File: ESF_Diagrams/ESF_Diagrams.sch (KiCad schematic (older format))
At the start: 37 parts, among them M1 Motor, M2 Motor, U2 AIR, U3 AIR

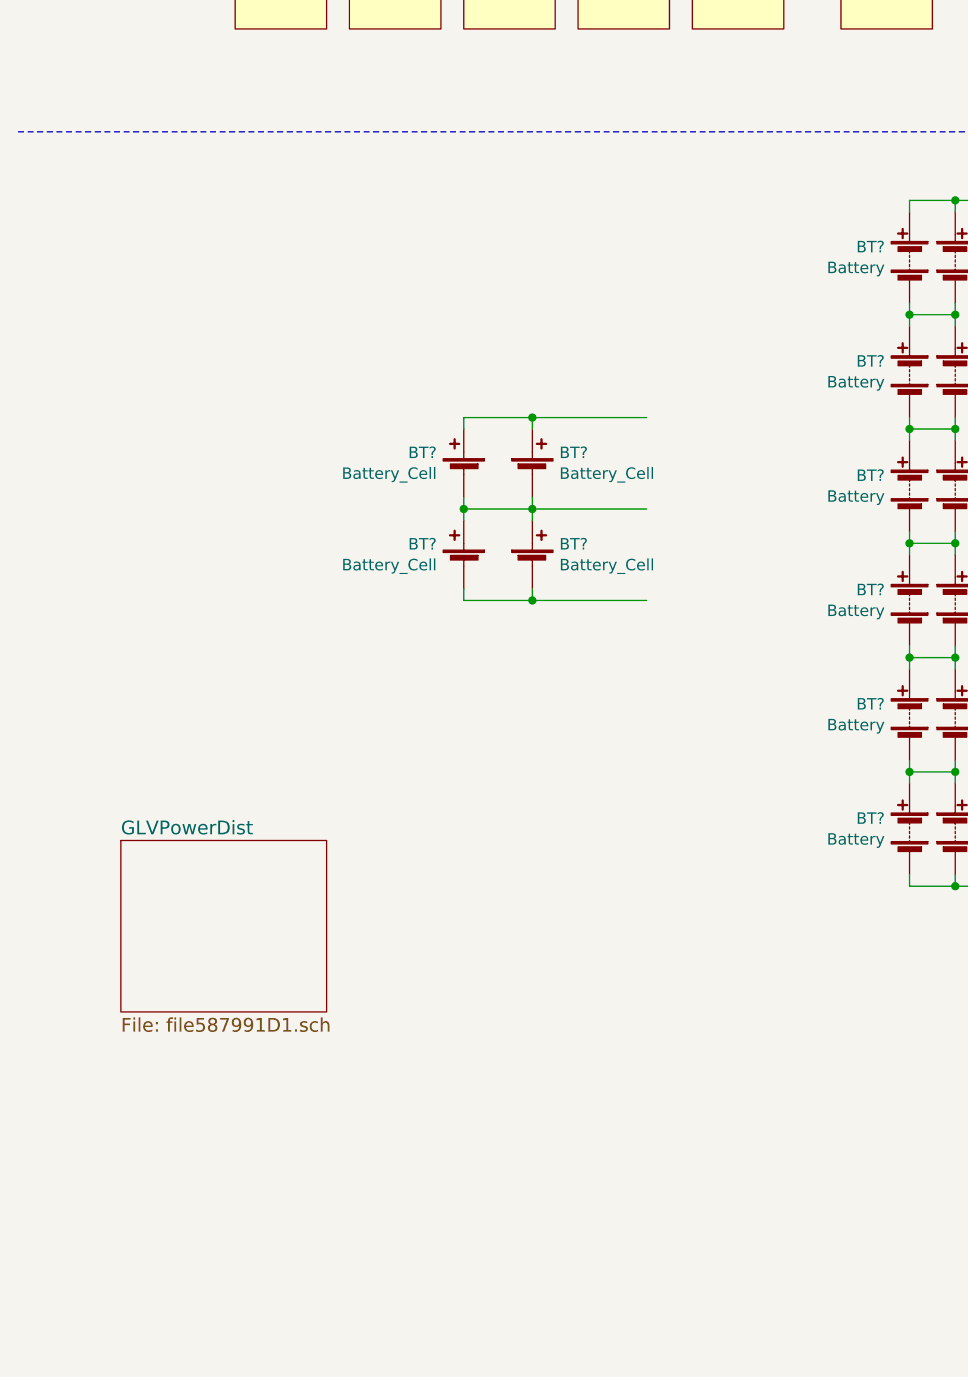
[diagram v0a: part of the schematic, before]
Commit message: Fix 2
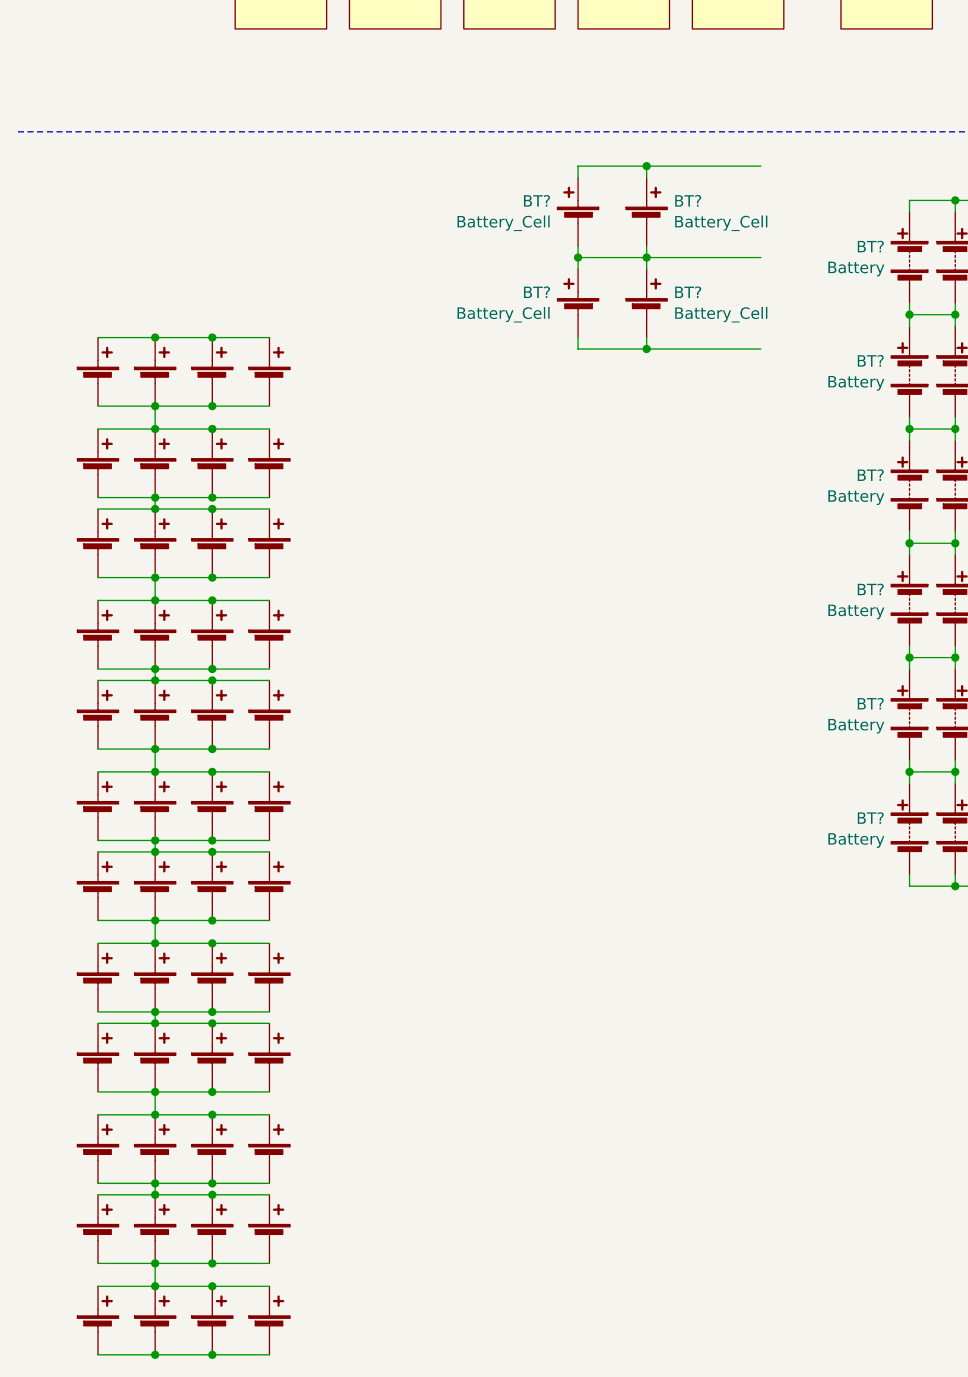
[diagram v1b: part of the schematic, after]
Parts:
- added BT? (x48): Battery_Cell, symbol Battery_Cell
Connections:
- wire segments 88 -> 123
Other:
- moved on the sheet: BT?
